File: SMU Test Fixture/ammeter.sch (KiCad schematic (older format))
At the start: 43 parts, among them K10 Integrator Reset, K5 3x Gain Enable, K6 Shunt Select, K7 Sense Select, K8 I/V Mode Select, K9 Shunt/Sense Select, U1 OPA189, U2 OPA551U, U3 OPA189, U4 OPA1611, U5 OPA192, U6 OPA192

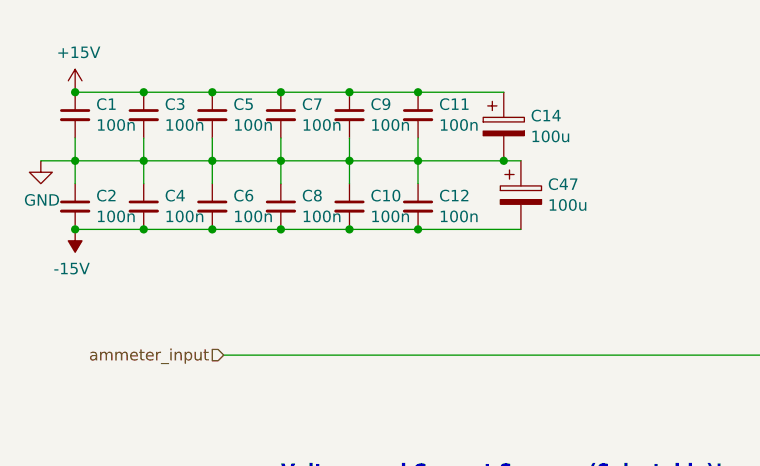
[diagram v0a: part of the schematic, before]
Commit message: Footprint updates
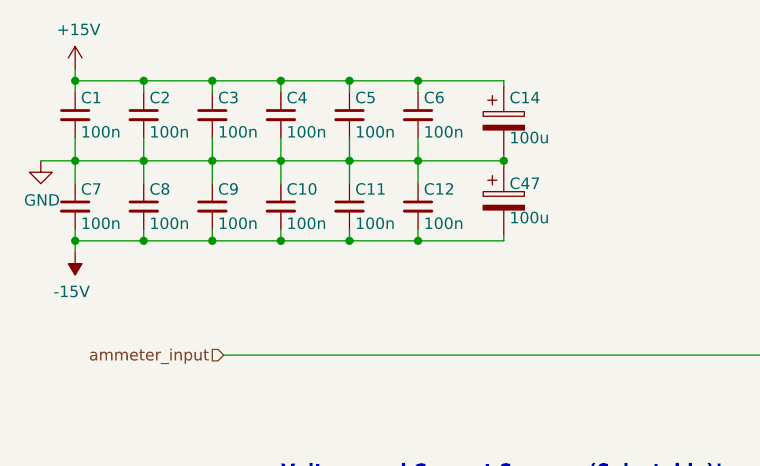
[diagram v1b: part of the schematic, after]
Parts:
- C1, C10, C11, C12, C2, C3, C4, C5, C6, C7, C8, C9: footprint Capacitor_SMD:C_0805_2012Metric_Pad1.18x1.45mm_HandSolder -> Capacitor_SMD:C_1206_3216Metric_Pad1.33x1.80mm_HandSolder; PN (none) -> CGA5L2C0G1H104J160AA
- C13: footprint Capacitor_SMD:C_0805_2012Metric_Pad1.18x1.45mm_HandSolder -> Capacitor_SMD:C_0201_0603Metric_Pad0.64x0.40mm_HandSolder; PN (none) -> GRM0335C1H330FA01D
- R10: PN (none) -> CRCW080556K0JNEA
- R12: PN (none) -> RQ73C2A11K8BTDF
- R16, R17: footprint Resistor_SMD:R_0805_2012Metric_Pad1.20x1.40mm_HandSolder -> Resistor_SMD:R_1206_3216Metric_Pad1.30x1.75mm_HandSolder; PN (none) -> RG3216N-1004-W-T1
- R18, R19: PN (none) -> CRCW08055K00JNTA
- R8: PN (none) -> RN73C2A5K9BTDF
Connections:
- net +15V: now also C2.1, C4.1, C6.1; no longer C11.1, C7.1, C9.1
- net -15V: now also C11.2, C7.2, C9.2; no longer C2.2, C4.2, C6.2
- net GND: now also C11.1, C2.2, C4.2, C6.2, C7.1, C9.1; no longer C11.2, C2.1, C4.1, C6.1, C7.2, C9.2
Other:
- moved on the sheet: C14, C47
